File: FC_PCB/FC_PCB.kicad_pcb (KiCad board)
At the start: 2 copper layers, 60 x 40 mm, 99 parts, among them IC1 ICM-42688-P, IC2 CAM-M8Q-0, IC3 BMP390, IC4 IIS2MDCTR, J1 PWM1, J3 USB_C_Receptacle_USB2.0_16P, J4 PWM2, J5 PWM3, J6 PWM4, J7 I2C, J8 UART, J9 SPI, Q1 EMH3, SW1 RESET, SW2 RESET, U1 ESP32-S3-MINI-1, U2 CP2102N-Axx-xQFN24, U3 TPS56339DDC, U4 TPS56339DDC, U5 INA226, U6 W25Q128JVS

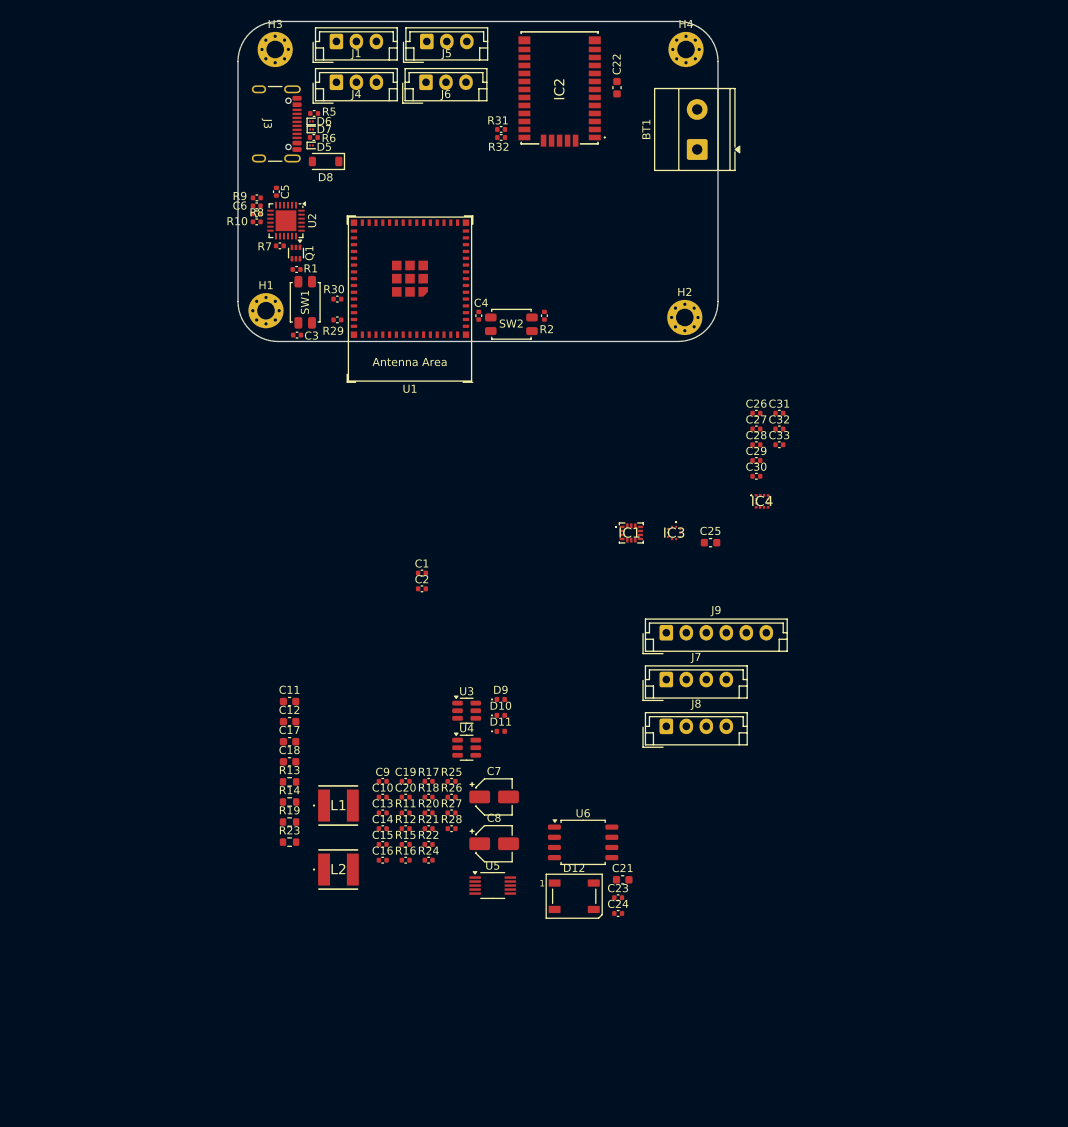
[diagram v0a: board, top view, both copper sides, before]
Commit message: Commit final hard
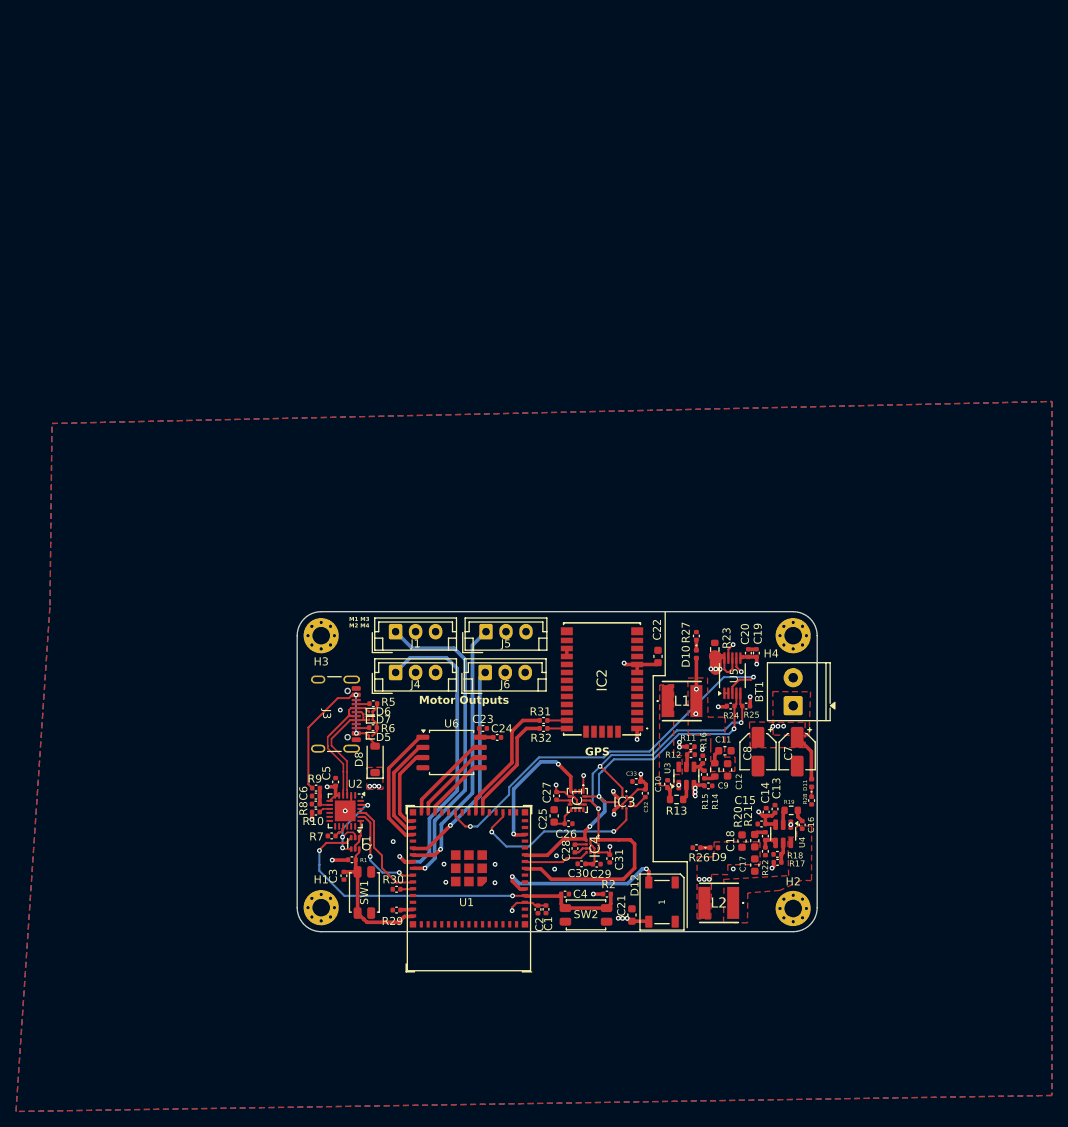
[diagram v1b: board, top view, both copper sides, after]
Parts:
- removed J7: I2C, Connector_JST:JST_EH_B4B-EH-A_1x04_P2.50mm_Vertical
- removed J8: UART, Connector_JST:JST_EH_B4B-EH-A_1x04_P2.50mm_Vertical
- removed J9: SPI, Connector_JST:JST_EH_B6B-EH-A_1x06_P2.50mm_Vertical
- added G***: LOGO, Library:logo, B.Cu at (116.9, 102.3)
- BT1: footprint TerminalBlock_Phoenix:TerminalBlock_Phoenix_MKDS-1,5-2_1x02_P5.00mm_Horizontal -> TerminalBlock_Phoenix:TerminalBlock_Phoenix_PT-1,5-2-3.5-H_1x02_P3.50mm_Horizontal
- R20: footprint Capacitor_SMD:C_0402_1005Metric -> Capacitor_SMD:C_0603_1608Metric
- moved H2 75.1 mm to (164.4, 125.9)
- moved D8 75.0 mm to (112.1, 107.2), turned to 90 degrees
- moved H1 74.9 mm to (105.4, 125.8)
- moved H4 74.5 mm to (164.4, 91.8)
- moved SW2 74.4 mm to (138.5, 126.7)
- moved C5 74.1 mm to (107.2, 110.1)
- moved C6 74.1 mm to (104.7, 111.8)
- moved D5 74.1 mm to (111.6, 104.3)
- moved D6 74.1 mm to (111.6, 101.3)
- moved D7 74.1 mm to (111.6, 102.3)
- moved J1 74.1 mm to (114.7, 91.3)
- moved J3 74.1 mm to (106.1, 101.6)
- moved J4 74.1 mm to (114.7, 96.4)
- moved J5 74.1 mm to (126.0, 91.3)
- moved J6 74.1 mm to (125.9, 96.4)
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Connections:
- J6 pad 1: /ESP_PERIPHE/ESC_PWM4 -> /ESP_MCU/ESC_PWM4
- U1 pad 10: /ESP_MCU/ESP_UART2_TX -> /ESP_ALIM/CS_I2C_SDA
- U1 pad 11: /ESP_MCU/ESP_UART2_RX -> unconnected-(U1-GPIO7/TOUCH7/ADC1_CH6-Pad11)
- U1 pad 12: /ESP_MCU/GPIO_8 -> unconnected-(U1-GPIO8/TOUCH8/ADC1_CH7/SUBSPICS1-Pad12)
- U1 pad 14: /ESP_MCU/ESP_SPI2_CS0 -> unconnected-(U1-GPIO10/TOUCH10/ADC1_CH9/FSPICS0/FSPIIO4/SUBSPICS0-Pad14)
- U1 pad 15: /ESP_MCU/ESP_SPI2_MOSI -> unconnected-(U1-GPIO11/TOUCH11/ADC2_CH0/FSPID/FSPIIO5/SUBSPID-Pad15)
- U1 pad 16: /ESP_MCU/ESP_SPI2_SCK -> unconnected-(U1-GPIO12/TOUCH12/ADC2_CH1/FSPICLK/FSPIIO6/SUBSPICLK-Pad16)
- U1 pad 17: /ESP_MCU/ESP_SPI2_MISO -> unconnected-(U1-GPIO13/TOUCH13/ADC2_CH2/FSPIQ/FSPIIO7/SUBSPIQ-Pad17)
- U1 pad 26: /ESP_ACTION/MEM_HOLD -> unconnected-(U1-GPIO26-Pad26)
- U1 pad 28: /ESP_ACTION/MEM_WP -> /ESP_ACTION/MEM_DI
- U1 pad 29: /ESP_ACTION/MEM_CS -> /ESP_ACTION/MEM_CLK
- U1 pad 30: unconnected-(U1-GPIO48/SPICLK_N/SUBSPICLK_N_DIFF-Pad30) -> /ESP_ACTION/MEM_HOLD
- U1 pad 31: /ESP_ACTION/MEM_DI -> /ESP_ACTION/MEM_WP
- U1 pad 32: /ESP_ACTION/MEM_CLK -> /ESP_ACTION/MEM_DO
- U1 pad 33: /ESP_ACTION/MEM_DO -> /ESP_ACTION/MEM_CS
- U1 pad 35: /ESP_MCU/ESC_PWM3 -> /ESP_MCU/ESC_PWM4
- U1 pad 8: /ESP_ALIM/CS_I2C_SDA -> /ESP_ALIM/CS_I2C_SCL
- U1 pad 9: /ESP_ALIM/CS_I2C_SCL -> /ESP_MCU/GPIO_8
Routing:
- net +5V: track 0.00 -> 108.0 mm, vias 0 -> 10
- net /ESP_ALIM/CS_I2C_SCL: track 0.00 -> 63.1 mm, vias 0 -> 3
- net /ESP_ALIM/CS_ALERT: track 0.00 -> 50.5 mm, vias 0 -> 2
- net /ESP_ALIM/V_ALIM: track 0.00 -> 50.0 mm, vias 0 -> 11
- net /ESP_MCU/BOOT: track 0.00 -> 48.0 mm, vias 0 -> 2
- net /ESP_ALIM/CS_I2C_SDA: track 0.00 -> 46.2 mm, vias 0 -> 3
- net +3.3V: track 0.00 -> 44.6 mm, vias 0 -> 16
- net /ESP_MCU/ESC_PWM2: track 0.00 -> 40.0 mm, vias 0 -> 1
- net /ESP_MCU/ESC_PWM1: track 0.00 -> 39.7 mm, vias 0 -> 1
- net /ESP_MCU/ESC_PWM3: track 0.00 -> 33.3 mm, vias 0 -> 1
- net /ESP_MCU/ESC_PWM4: track 0.00 -> 26.8 mm, vias 0 -> 1
- net GND: track 0.00 -> 24.0 mm, vias 0 -> 18
- net /ESP_MCU/VBUS: track 0.00 -> 23.6 mm, vias 0 -> 2
- net /ESP_MCU/GPIO_14: track 0.00 -> 23.4 mm, vias 0 -> 2
- net /ESP_ACTION/RGB_PIN: track 0.00 -> 22.3 mm, vias 0 -> 2
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- added copper zone on F.Cu, net +3.3V
- added copper zone on In2.Cu, net +3.3V
- added copper zone on F.Cu, net +5V
- added copper zone on F.Cu, net /ESP_ALIM/V_ALIM
- added copper zone on B.Cu, net GND
- added copper zone on F.Cu, net GND
- added copper zone on In1.Cu, net GND
- added copper zone on F.Cu, net Net-(U3-BOOT)
- added copper zone on F.Cu, net Net-(U4-BOOT)
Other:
- board size 60 x 40 mm -> 65 x 40 mm
- copper layers 2 -> 4
- board text added: "FC-GAOL-1"
- board text added: "GPS"
- board text added: "M1 M3 M2 M4"
- board text added: "Motor Outputs"
